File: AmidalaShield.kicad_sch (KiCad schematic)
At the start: 1 part

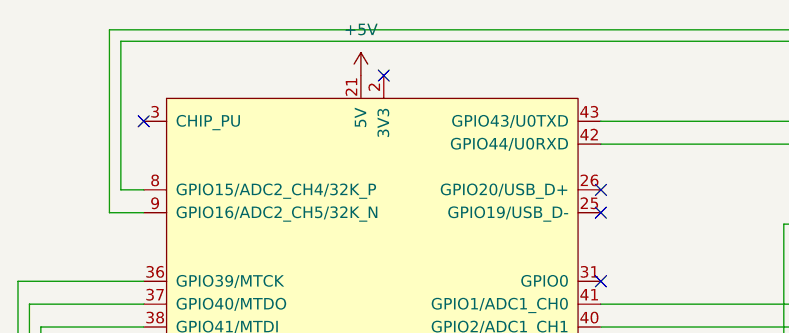
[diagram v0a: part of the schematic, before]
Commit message: Updated to v1.2 to address remaining issues
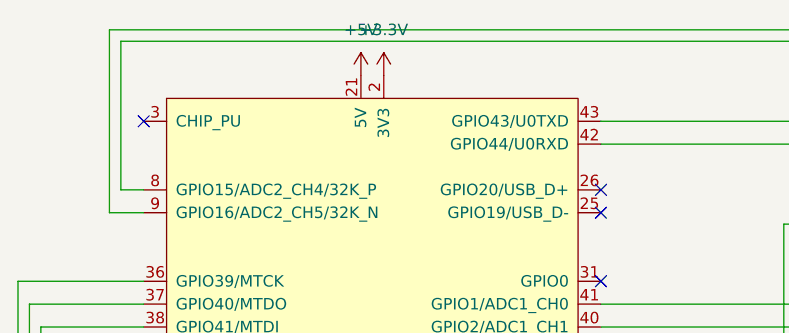
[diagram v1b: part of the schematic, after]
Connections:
- net +3.3V: now reaches ESP32-S3.1 (3V3), ESP32-S3.2 (3V3)
- no-connect marks 11 -> 10
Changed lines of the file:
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@@
-	)
-	(no_connect
-		(at 55.88 22.86)
 	)
 	(no_connect
@@
 		)
 	)
+	(symbol
+		(lib_id "power:+3.3V")
+		(at 55.88 22.86 0)
+		(unit 1)
+		(exclude_from_sim no)
+		(in_bom yes)
+		(on_board yes)
+		(dnp no)
+		(fields_autoplaced yes)
+		(property "Reference" "#PWR023"
+			(at 55.88 26.67 0)
+			(effects
+				(font
+					(size 1.27 1.27)
+				)
+				(hide yes)
+			)
+		)
+		(property "Value" "+3.3V"
+			(at 55.88 17.78 0)
+			(effects
+				(font
+					(size 1.27 1.27)
+				)
+			)
+		)
+		(property "Footprint" ""
+			(at 55.88 22.86 0)
+			(effects
+				(font
+					(size 1.27 1.27)
+				)
+				(hide yes)
+			)
+		)
+		(property "Datasheet" ""
+			(at 55.88 22.86 0)
+			(effects
+				(font
+					(size 1.27 1.27)
+				)
+				(hide yes)
+			)
+		)
+		(property "Description" "Power symbol creates a global label with name \"+3.3V\""
+			(at 55.88 22.86 0)
+			(effects
+				(font
+					(size 1.27 1.27)
+				)
+				(hide yes)
+			)
+		)
+		(pin "1"
+		)
+		(instances
+			(project "AmidalaShield"
+				(path "/6d8d0000-f03d-4277-95db-0f566c3960c4"
+					(reference "#PWR023")
+					(unit 1)
+				)
+			)
+		)
+	)
